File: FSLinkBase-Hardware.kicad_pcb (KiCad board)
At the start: 4 copper layers, 30 x 13.5 mm, 45 parts, among them J1 USB_C_Receptacle_USB2.0, J2 Conn_02x05_Counter_Clockwise, U1 ESD0524P, U2 CH32X035F8U6, U3 TTP233H-RB6, U4 TTP233H-RB6, U5 RS2227XUTQK10, U6 RS2227XUTQK10, U7 TPS25200, U8 RT8010

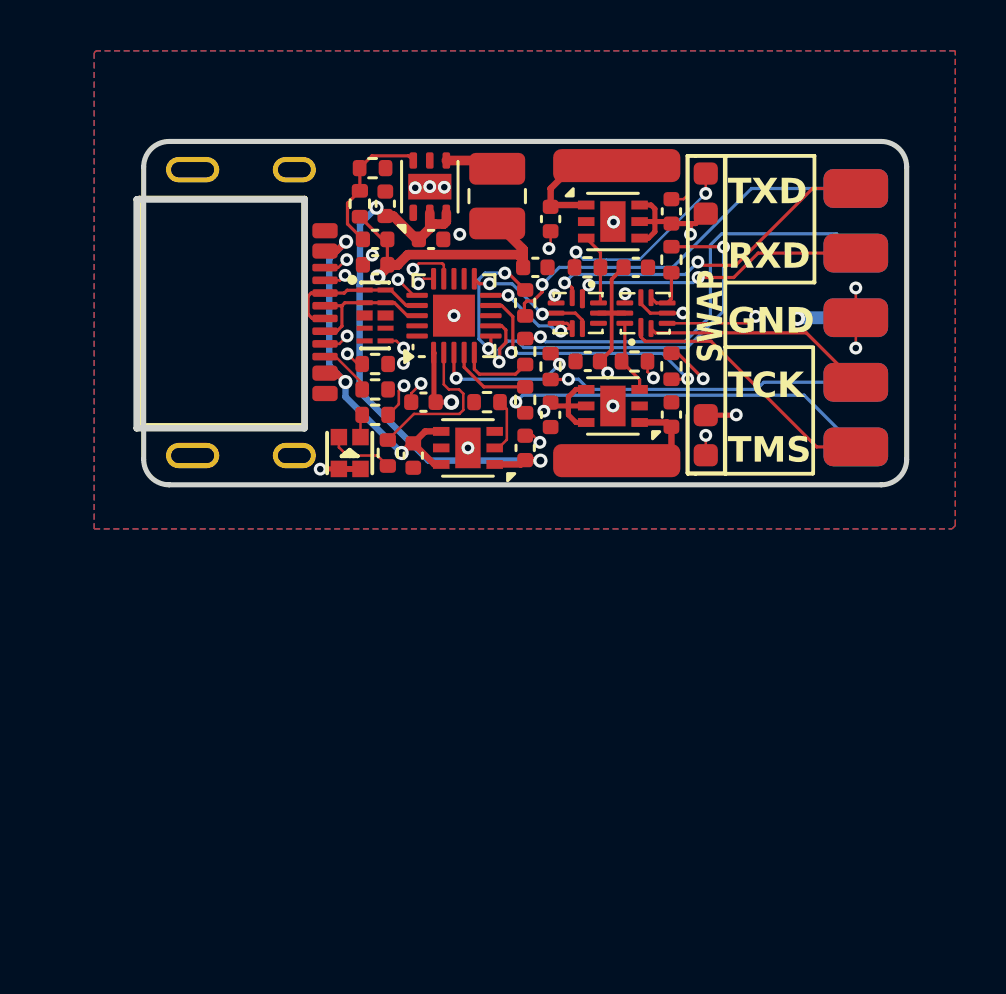
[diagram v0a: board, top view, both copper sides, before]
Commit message: update
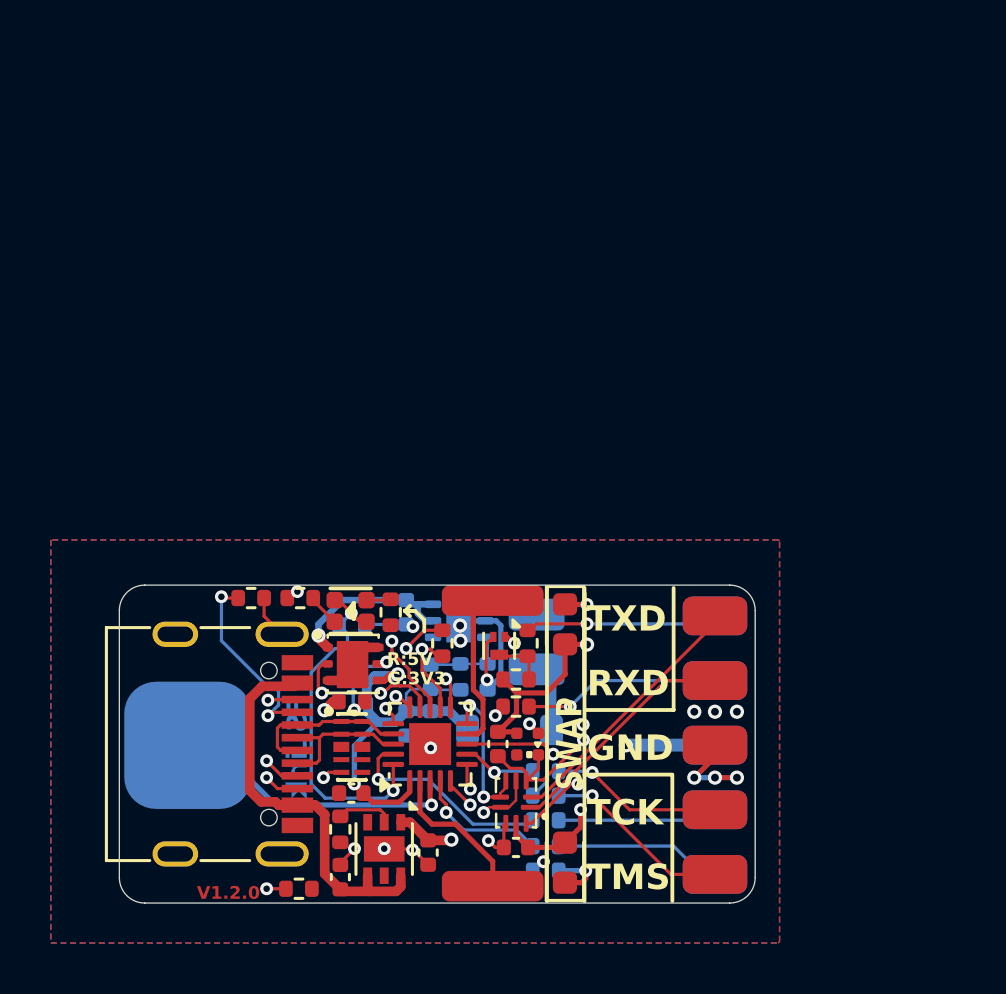
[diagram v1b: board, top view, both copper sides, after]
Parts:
- removed C13, C4, C5, C6: 0.1u, Capacitor_SMD:C_0402_1005Metric
- removed C3: 50p, Capacitor_SMD:C_0402_1005Metric
- removed D1: XL-1615SURUGC, MyLED:LED-SMD_4P-L1.6-W1.5-TL-1
- removed U3, U4: TTP233H-RB6, Package_DFN_QFN:DFN-6-1EP_2x2mm_P0.65mm_EP1x1.6mm
- removed U5: RS2227XUTQK10, My DFN_QFN:WQFN-10_L1.8-W1.4-P0.40-BL
- added D2: LED, LED_SMD:LED_0603_1608Metric, F.Cu at (61.6, 45.6)
- added D5: SS24, Diode_SMD:D_SOD-123, B.Cu at (59.4, 49.8)
- added D7: XL-1615SURUGC, MyLED:LED-SMD_4P-L1.6-W1.5-TL-1, F.Cu at (53.1, 45.1)
- added Q1: HSCB20D03, My DFN_QFN:DFN-6_L2.0-W2.0-P0.65-BL-EP2, F.Cu at (53.2, 47.2)
- added Q2: 2N7002, Package_DFN_QFN:Diodes_DFN1006-3, B.Cu at (53.2, 46.9)
- added Q3: 2N7002, Package_DFN_QFN:Diodes_DFN1006-3, F.Cu at (59.0, 46.5)
- added R16: 5.1k, Resistor_SMD:R_0402_1005Metric, F.Cu at (56.7, 46.4)
- added R17: 5.1k, Resistor_SMD:R_0402_1005Metric, B.Cu at (60.8, 55.3)
- added R18: 22R, Resistor_SMD:R_0402_1005Metric, F.Cu at (60.1, 46.4)
- added TP3: TouchPad, Touch Pad:Touch_SMD_BOX_5.0x5.0mm, B.Cu at (46.7, 50.3)
- C12, C14, C8, C9, L1, R10, R13, R14, R5, R6, R9, U8: moved to B.Cu
- C2: value 50p -> 0.1u
- D4: value LED -> WS2812; footprint LED_SMD:LED_0603_1608Metric -> MyLED:LED-SMD_4P-L1.0-W1.0-TL_XL-1010RGBC-WS2812B
- J1: footprint My USB Connector:USB-C-SMD_SHOU_TYPE-C-16P-CB1.6 -> Connector_USB:USB_C_Receptacle_G-Switch_GT-USB-7010ASV
- R3: value 1k -> 10k
- R4: value 1k -> 100k; moved to B.Cu
- R8: value 22R -> 10k
- TP1, TP2: footprint Touch Pad:Touch_SMD_BOX -> Touch Pad:Touch_SMD_BOX_1.2x4.0mm
- moved R6 23.6 mm to (60.8, 54.4), turned to 0 degrees
- moved C7 23.3 mm to (59.6, 54.4), turned to 180 degrees
- moved D4 22.7 mm to (60.1, 50.3), turned to 90 degrees
- moved R14 20.5 mm to (58.5, 47.7), turned to -90 degrees
- moved R2 19.9 mm to (51.1, 56.0)
- moved U6 19.4 mm to (59.6, 52.6), turned to 90 degrees
- moved R13 19.0 mm to (57.5, 47.7)
- moved C14 18.6 mm to (55.3, 49.5), turned to -90 degrees
- moved R5 18.5 mm to (60.8, 53.3), turned to 180 degrees
- moved C9 18.2 mm to (56.3, 49.5), turned to -90 degrees
- moved TP2 17.8 mm to (58.7, 44.7)
- moved R15 17.8 mm to (52.7, 53.7), turned to -90 degrees
- moved J2 17.7 mm to (67.5, 55.5)
- moved D3 17.7 mm to (61.6, 55.0)
- moved L1 17.6 mm to (60.5, 46.3)
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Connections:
- C1 pad 1: +3V3 -> VCC
- C14 pad 1: +3V3 -> VCC
- C2 pad 1: Net-(U3-I) -> VCC
- C7 pad 1: +3V3 -> VCC
- C8 pad 1: +3V3 -> VCC
- C9 pad 1: +3V3 -> VCC
- D3 pad 2: +3V3 -> VCC
- D4 pad 1: Net-(D4-K) -> VCC
- D4 pad 2: +3V3 -> unconnected-(D4-DOUT-Pad2)
- J1 pad A8: /SWCLK -> /SWDIO
- J1 pad B8: /SWDIO -> /SWCLK
- J2 pad 1: /R_TMS -> /TMS
- J2 pad 2: /R_TCK -> /TCK
- J2 pad 8: +3V3 -> VCC
- L1 pad 1: +3V3 -> Net-(D5-A)
- R10 pad 1: Net-(U2-PA1) -> Net-(U2-PA6)
- R10 pad 2: /TDI -> /TMS
- R11 pad 2: /LED1 -> GND
- R12 pad 1: Net-(D1-K2) -> VCC
- R12 pad 2: /LED2 -> Net-(D7-A2)
- R13 pad 1: +3V3 -> VCC
- R3 pad 1: /SWAP_SWD -> +5V
- R3 pad 2: Net-(D3-K) -> Net-(Q1A-G)
- R4 pad 1: /SWAP_UART -> /SWAP_PW
- R4 pad 2: Net-(D4-K) -> GND
- R5 pad 1: Net-(U2-PA7) -> /TDI
- R5 pad 2: /TMS -> Net-(U2-PC14)
- R6 pad 1: Net-(U2-PA5) -> Net-(U2-PA2)
- R6 pad 2: /TCK -> /TDO
- R7 pad 1: Net-(U2-PA4) -> Net-(U2-PA3)
- R7 pad 2: /SRST -> /TRST
- R8 pad 1: Net-(U2-PA3) -> VCC
- R8 pad 2: /TRST -> Net-(Q3-D)
- R9 pad 1: Net-(U2-PA2) -> Net-(U2-PA5)
- R9 pad 2: /TDO -> /TCK
- TP1 pad 1: Net-(U3-I) -> /TK_S
- TP2 pad 1: Net-(U4-I) -> /TK_U
- U2 pad 1: +3V3 -> VCC
- U2 pad 12: unconnected-(U2-PB3-Pad12) -> /SWAP_UART
- U2 pad 13: unconnected-(U2-PB11-Pad13) -> /SWAP_SWD
- U2 pad 15: /LED2 -> /WS2812
- U2 pad 19: unconnected-(U2-PC14-Pad19) -> Net-(U2-PC14)
- U2 pad 2: /LED1 -> /TK_S
- U2 pad 20: unconnected-(U2-PC15-Pad20) -> /SWAP_PW
- U2 pad 3: Net-(U2-PA1) -> /TK_P
- U2 pad 6: Net-(U2-PA4) -> /RST
- U2 pad 8: unconnected-(U2-PA6-Pad8) -> Net-(U2-PA6)
- U2 pad 9: Net-(U2-PA7) -> /TK_U
- U6 pad 9: +3V3 -> VCC
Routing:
- net +3V3: track 74.0 -> 0.00 mm, vias 8 -> 0
- net VCC: track 0.00 -> 58.6 mm, vias 0 -> 6
- net /SWAP_UART: track 2.81 -> 25.7 mm, vias 0 -> 2
- net /SWAP_SWD: track 2.95 -> 20.6 mm, vias 0 -> 2
- net /SWAP_PW: track 0.00 -> 14.9 mm, vias 0 -> 2
- net GND: track 11.6 -> 25.9 mm, vias 19 -> 18
- net Net-(U2-PA5): track 16.7 -> 2.90 mm, vias 2 -> 1
- net /RST: track 0.00 -> 12.7 mm, vias 0 -> 2
- net /SWDIO: track 6.11 -> 17.1 mm
- net /TK_P: track 0.00 -> 10.9 mm, vias 0 -> 1
- net Net-(D2-K): track 0.00 -> 10.9 mm, vias 0 -> 2
- net /R_TMS: track 10.6 -> 0.00 mm
- net Net-(U2-PA7): track 10.5 -> 0.00 mm, vias 2 -> 0
- net /WS2812: track 0.00 -> 9.11 mm, vias 0 -> 2
- net /TRST: track 16.8 -> 7.74 mm
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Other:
- board size 30 x 13.5 mm -> 25 x 12.5 mm
- board text added: "FSLink"
- board text added: "G:3V3"
- board text added: "R:5V"
- board text added: "V1.2.0"
- board text added: "VCC"
- board text removed: "3V3"
